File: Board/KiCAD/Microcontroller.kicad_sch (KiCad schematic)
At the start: 29 parts, among them J2 Conn_ARM_SWD_TagConnect_TC2030, J4 Conn_01x03, SW2 SW_Push, U5 LMR50410, U9 STM32F103C8T6, Y1 Crystal_GND24_Small, Y4 CM8V-T1A-32.768KHZ-12.5PF-20P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

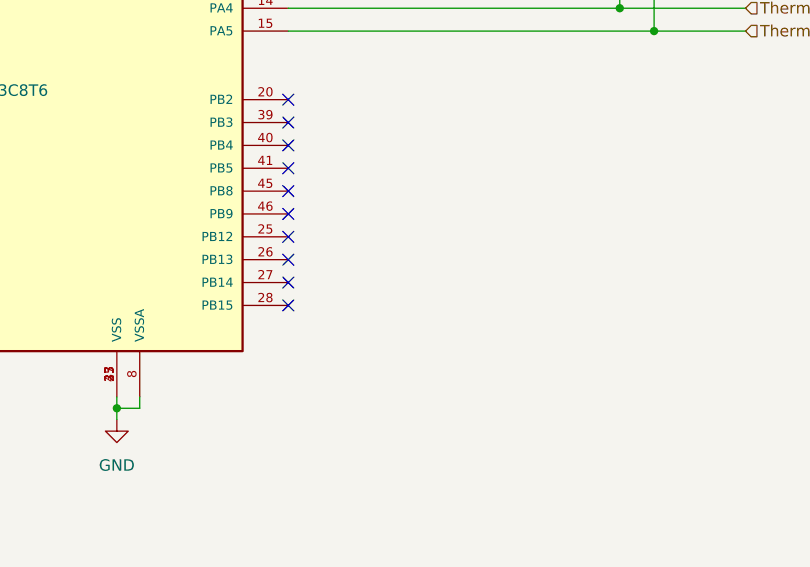
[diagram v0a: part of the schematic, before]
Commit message: EPL - Battery Management System REV 2
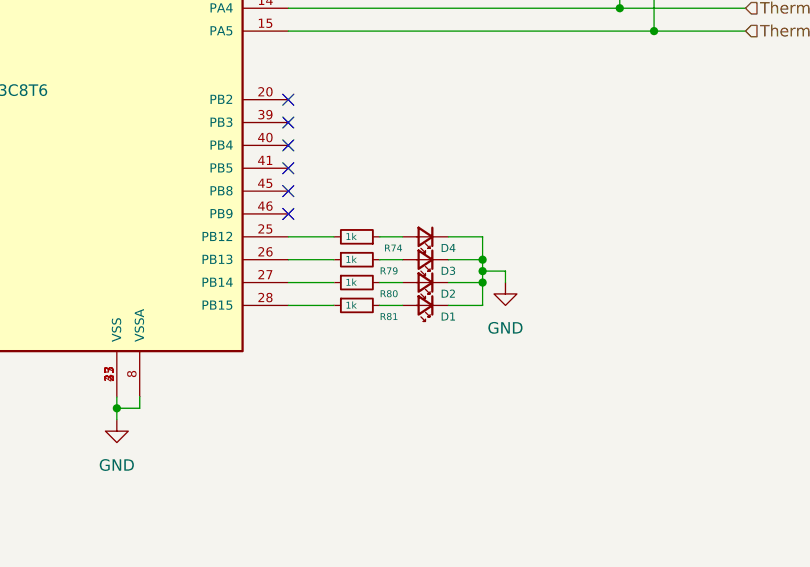
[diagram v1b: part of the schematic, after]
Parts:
- added D1, D2, D3, D4: LED_Small, LED_SMD:LED_0603_1608Metric, symbol Device:LED_Small
- added R74, R79, R80, R81: 1k, Resistor_SMD:R_0603_1608Metric, symbol Device:R_Small
- SW2: footprint Button_Switch_SMD:SW_Push_1P1T_NO_CK_KMR2 -> Button_Switch_SMD:SW_Push_SPST_NO_Alps_SKRK
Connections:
- net GND: now also D1.1 (K), D2.1 (K), D3.1 (K), D4.1 (K)
- net at U9.25 (PB12): now also R74.2
- net at U9.26 (PB13): now also R79.1
- net at U9.27 (PB14): now also R80.1
- net at U9.28 (PB15): now also R81.1
- new net: D3.2 (A), R79.2
- new net: D2.2 (A), R80.2
- new net: D4.2 (A), R74.1
- new net: D1.2 (A), R81.2
- no-connect marks 16 -> 12
